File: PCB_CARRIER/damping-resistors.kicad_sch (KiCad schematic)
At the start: 32 parts

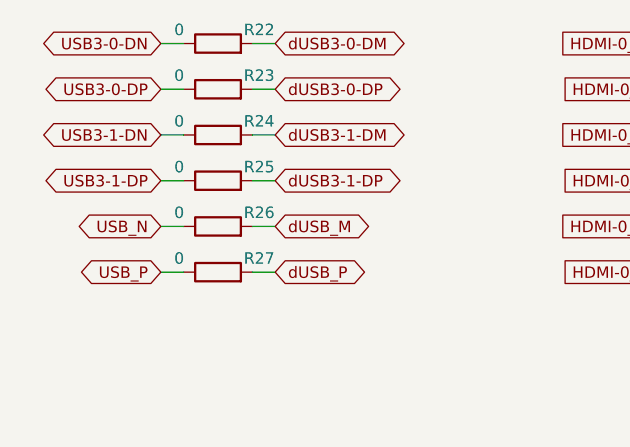
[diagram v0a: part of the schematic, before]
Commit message: added USB 2 netclass
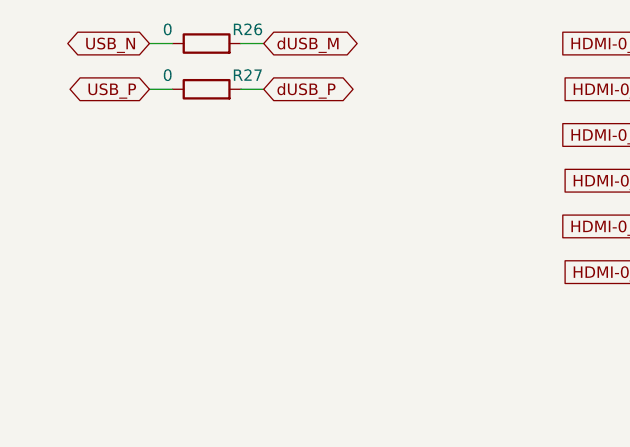
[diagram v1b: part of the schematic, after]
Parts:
- removed R22, R23, R24, R25: 0, Resistor_SMD:R_0402_1005Metric, symbol Device:R
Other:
- moved on the sheet: R26, R27
